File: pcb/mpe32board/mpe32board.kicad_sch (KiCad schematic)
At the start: 42 parts, among them J1 Conn_ST_STDC14, J2 USB_C_Receptacle_USB2.0_16P, J46 Conn_02x10_Counter_Clockwise, SW1 SW_Push, SW2 SW_Push, U10 W9812G6KH-75, U2 USBLC6-2P6, U3 AMS1117-3.3, U9 STM32H743IITx

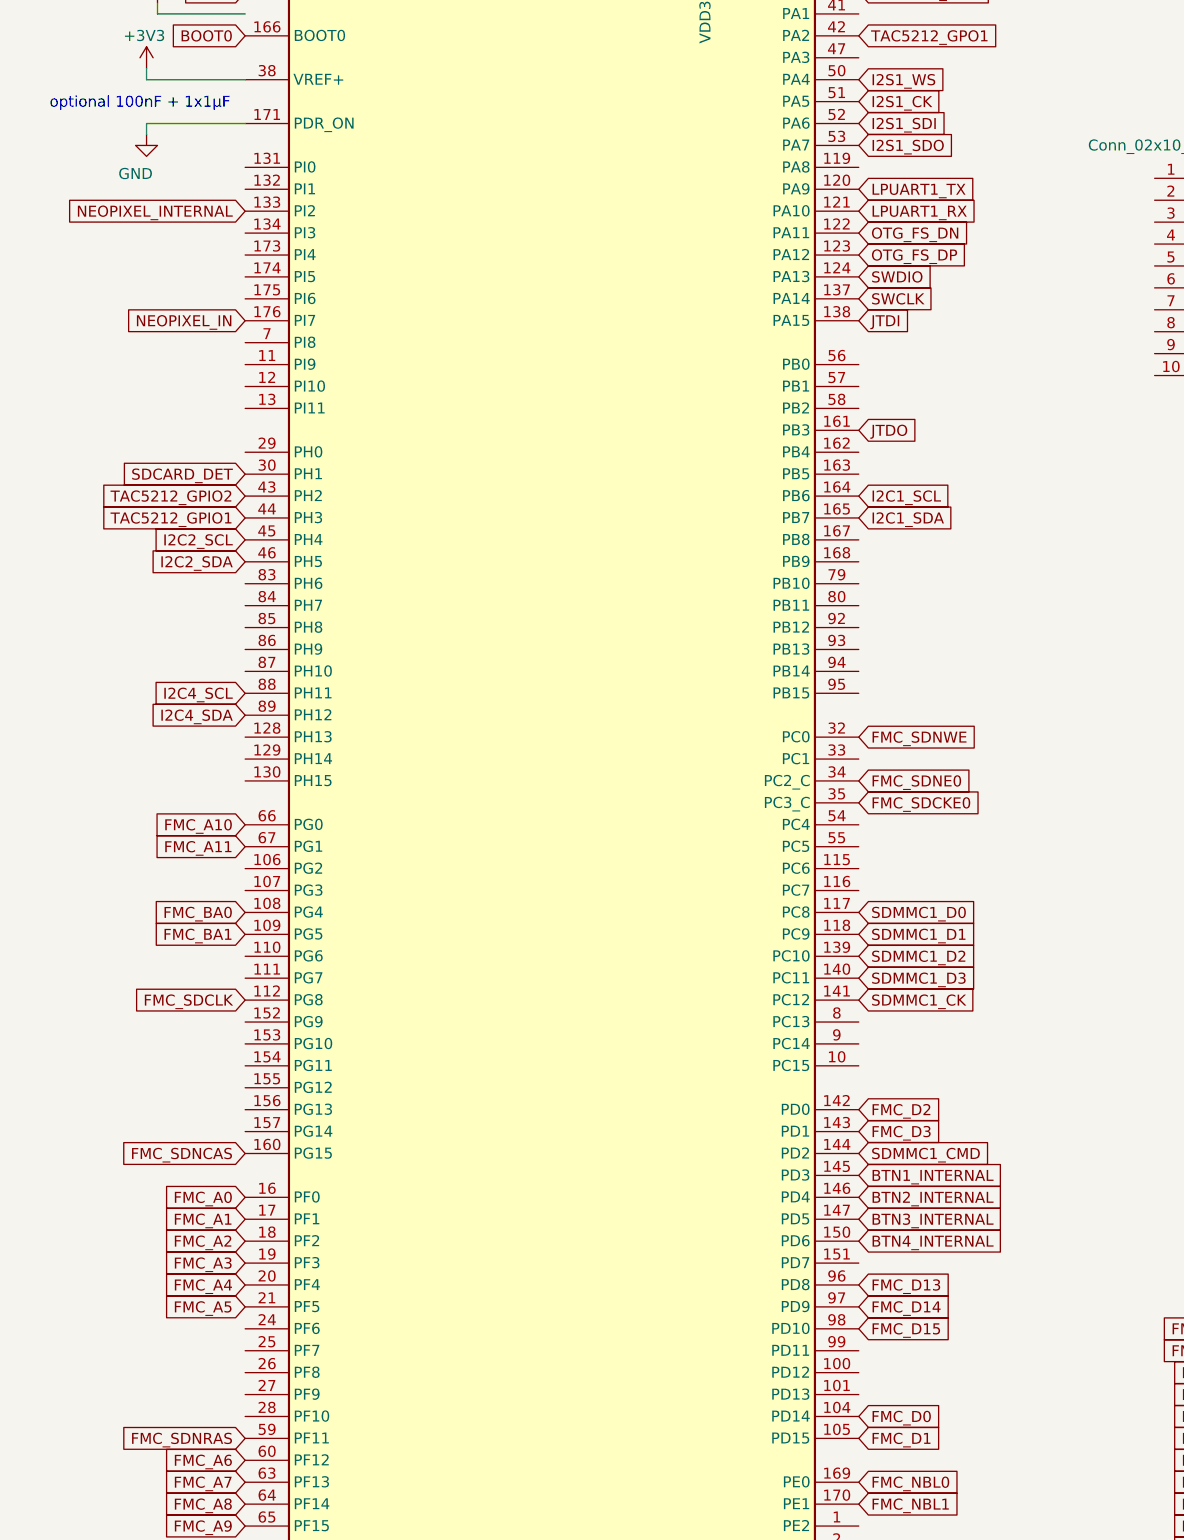
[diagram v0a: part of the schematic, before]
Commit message: route connectors
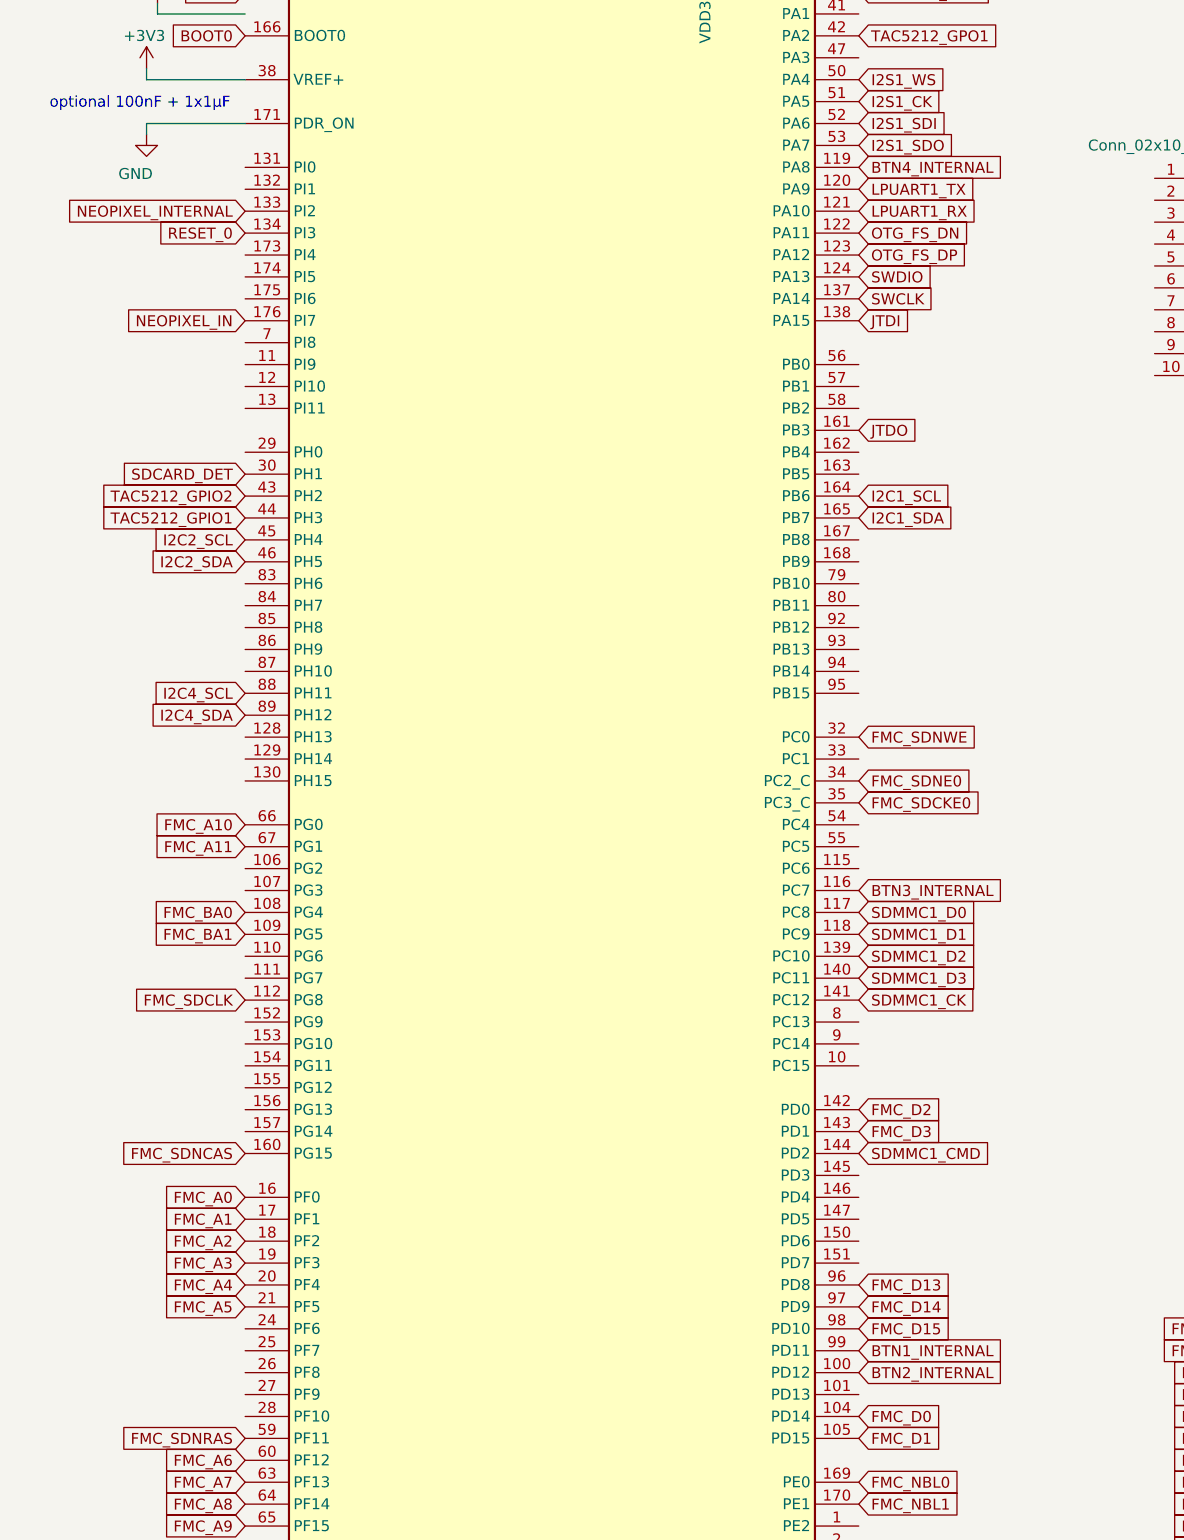
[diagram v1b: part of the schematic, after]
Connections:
- net BTN1_INTERNAL: now also U9.99 (PD11); no longer U9.145 (PD3)
- net BTN2_INTERNAL: now also U9.100 (PD12); no longer U9.146 (PD4)
- net BTN3_INTERNAL: now also U9.116 (PC7); no longer U9.147 (PD5)
- net BTN4_INTERNAL: now also U9.119 (PA8); no longer U9.150 (PD6)
- net RESET_0: now reaches U9.134 (PI3)
